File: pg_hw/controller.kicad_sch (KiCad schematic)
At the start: 33 parts, among them J1 USB_C_Receptacle_USB2.0_14P, Q1 SS8050, Q2 SS8050, SW1 SW_MEC_5E, SW2 SW_MEC_5E, U1 BW16, U2 AMS1117-3.3, U3 CH340C, U7 PCF8574A

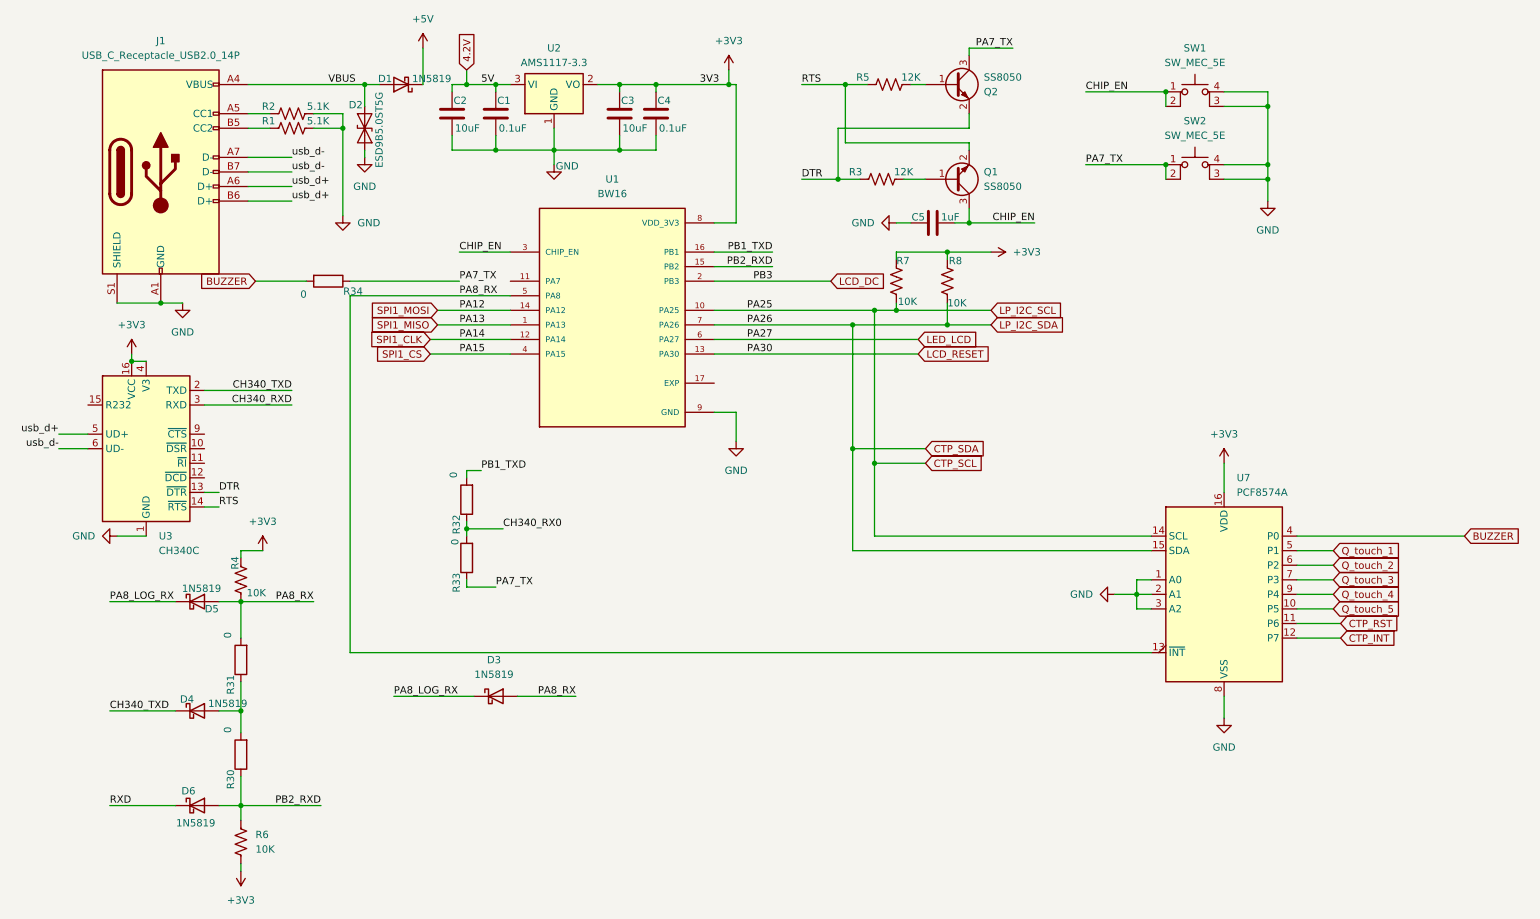
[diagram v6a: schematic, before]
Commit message: charlotte andeh
charlotte andeh
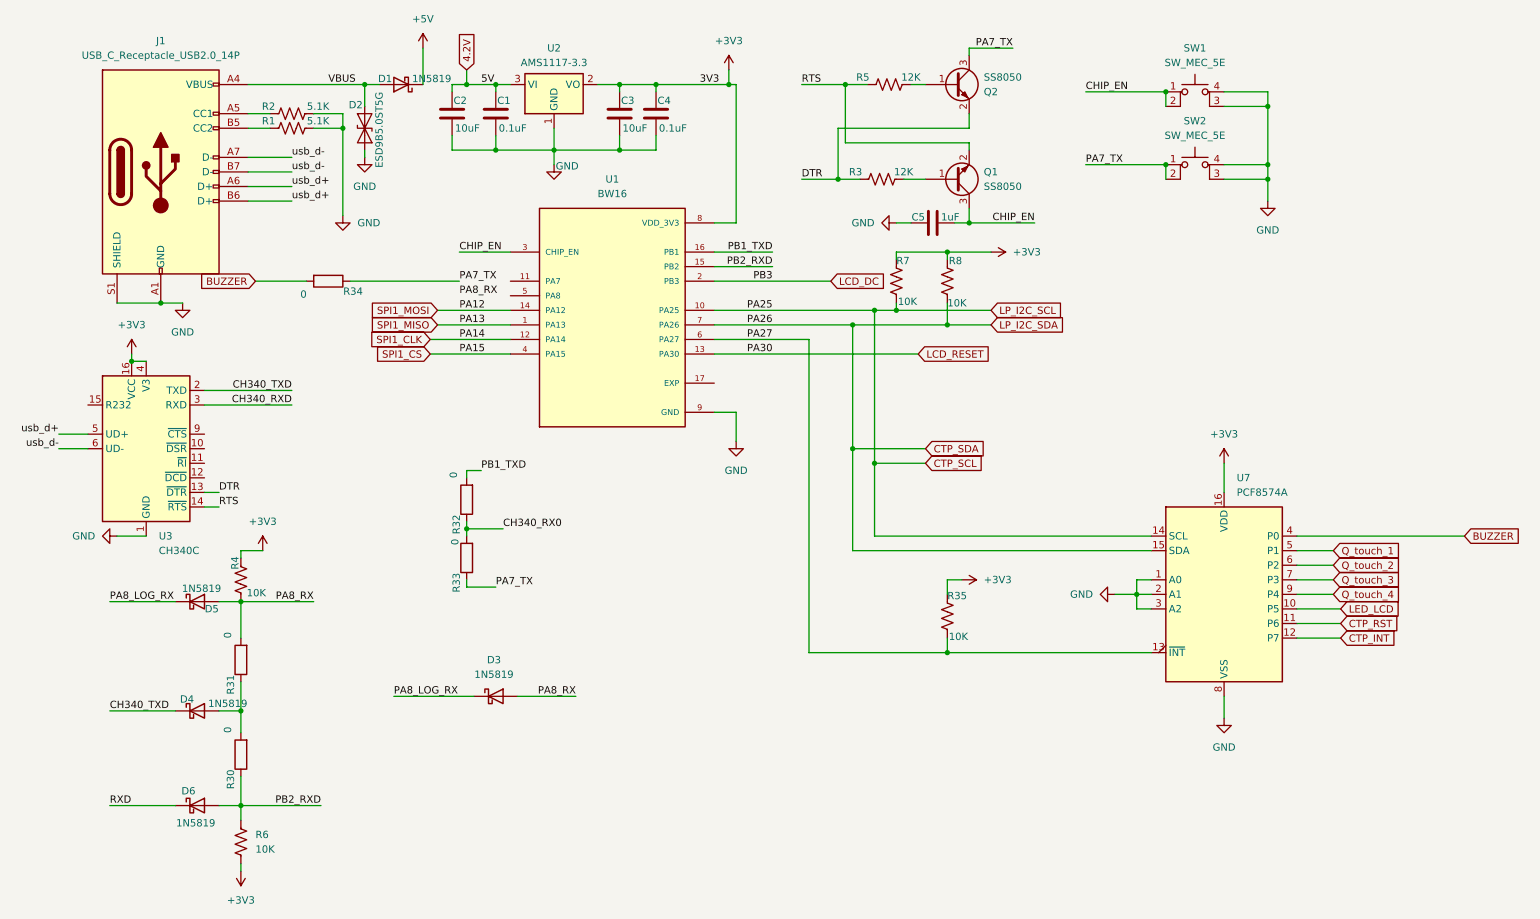
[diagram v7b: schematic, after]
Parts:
- added R35: 10K, Resistor_SMD:R_0402_1005Metric, symbol Device:R_US
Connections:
- net Q_touch_5 is gone; now on net LED_LCD: U7.10 (P5)
- net +3V3: now also R35.1
- net LED_LCD: no longer U1.6 (PA27)
- net PA8_RX: no longer U1.5 (PA8), U7.13 (~{INT})
- new net PA27: R35.2, U1.6 (PA27), U7.13 (~{INT})
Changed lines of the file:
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@@
 	)
 	(junction
+		(at 177.8 130.81)
+		(diameter 0)
+		(color 0 0 0 0)
+	)
+	(junction
 		(at 177.8 60.96)
 		(diameter 0)
@@
 	(wire
 		(pts
-			(xy 137.16 76.2) (xy 172.72 76.2)
+			(xy 137.16 76.2) (xy 153.67 76.2)
 		)
 		(stroke
@@
 	(wire
 		(pts
-			(xy 213.36 130.81) (xy 73.66 130.81)
-		)
-		(stroke
-			(width 0)
-			(type default)
-		)
-	)
-	(wire
-		(pts
 			(xy 201.93 45.72) (xy 215.9 45.72)
 		)
@@
 	(wire
 		(pts
-			(xy 73.66 130.81) (xy 73.66 68.58)
-		)
-		(stroke
-			(width 0)
-			(type default)
-		)
-	)
-	(wire
-		(pts
 			(xy 210.82 118.11) (xy 213.36 118.11)
 		)
@@
 	(wire
 		(pts
+			(xy 180.34 118.11) (xy 177.8 118.11)
+		)
+		(stroke
+			(width 0)
+			(type default)
+		)
+	)
+	(wire
+		(pts
 			(xy 93.98 109.22) (xy 100.33 109.22)
 		)
@@
 	(wire
 		(pts
-			(xy 238.76 123.19) (xy 245.11 123.19)
+			(xy 238.76 123.19) (xy 246.38 123.19)
 		)
 		(stroke
@@
 	(wire
 		(pts
+			(xy 177.8 128.27) (xy 177.8 130.81)
+		)
+		(stroke
+			(width 0)
+			(type default)
+		)
+	)
+	(wire
+		(pts
 			(xy 54.61 152.4) (xy 54.61 157.48)
 		)
@@
 	(wire
 		(pts
-			(xy 96.52 99.06) (xy 93.98 99.06)
+			(xy 153.67 130.81) (xy 153.67 76.2)
 		)
 		(stroke
@@
 	(wire
 		(pts
-			(xy 54.61 140.97) (xy 54.61 144.78)
+			(xy 96.52 99.06) (xy 93.98 99.06)
 		)
 		(stroke
@@
 	(wire
 		(pts
-			(xy 73.66 68.58) (xy 101.6 68.58)
+			(xy 54.61 140.97) (xy 54.61 144.78)
 		)
 		(stroke
@@
 	(wire
 		(pts
+			(xy 177.8 118.11) (xy 177.8 120.65)
+		)
+		(stroke
+			(width 0)
+			(type default)
+		)
+	)
+	(wire
+		(pts
 			(xy 109.22 43.18) (xy 120.65 43.18)
 		)
@@
 	(wire
 		(pts
+			(xy 177.8 130.81) (xy 153.67 130.81)
+		)
+		(stroke
+			(width 0)
+			(type default)
+		)
+	)
+	(wire
+		(pts
 			(xy 181.61 25.4) (xy 181.61 26.67)
 		)
@@
 	(wire
 		(pts
+			(xy 213.36 130.81) (xy 177.8 130.81)
+		)
+		(stroke
+			(width 0)
+			(type default)
+		)
+	)
+	(wire
+		(pts
 			(xy 171.45 31.75) (xy 173.99 31.75)
 		)
@@
 		)
 	)
-	(global_label "Q_touch_5"
-		(shape input)
-		(at 245.11 123.19 0)
-		(fields_autoplaced yes)
-		(effects
-			(font
-				(size 1.27 1.27)
-			)
-			(justify left)
-		)
-		(property "Intersheetrefs" "${INTERSHEET_REFS}"
-			(at 257.8317 123.19 0)
-			(effects
-				(font
-					(size 1.27 1.27)
-				)
-				(justify left)
-				(hide yes)
-			)
-		)
-	)
 	(global_label "CTP_INT"
 		(shape input)
@@
 	(global_label "LED_LCD"
 		(shape input)
-		(at 172.72 76.2 0)
+		(at 246.38 123.19 0)
 		(fields_autoplaced yes)
 		(effects
@@
 		)
 		(property "Intersheetrefs" "${INTERSHEET_REFS}"
-			(at 183.688 76.2 0)
+			(at 257.348 123.19 0)
 			(effects
 				(font
@@
 	)
 	(symbol
+		(lib_id "Device:R_US")
+		(at 177.8 124.46 0)
+		(unit 1)
+		(exclude_from_sim no)
+		(in_bom yes)
+		(on_board yes)
+		(dnp no)
+		(property "Reference" "R35"
+			(at 177.8 120.904 0)
+			(effects
+				(font
+					(size 1.27 1.27)
+				)
+				(justify left)
+			)
+		)
+		(property "Value" "10K"
+			(at 178.054 128.016 0)
+			(effects
+				(font
+					(size 1.27 1.27)
+				)
+				(justify left)
+			)
+		)
+		(property "Footprint" "Resistor_SMD:R_0402_1005Metric"
+			(at 178.816 124.714 90)
+			(effects
+				(font
+					(size 1.27 1.27)
+				)
+				(hide yes)
+			)
+		)
+		(property "Datasheet" "~"
+			(at 177.8 124.46 0)
+			(effects
+				(font
+					(size 1.27 1.27)
+				)
+				(hide yes)
+			)
+		)
+		(property "Description" "Resistor, US symbol"
+			(at 177.8 124.46 0)
+			(effects
+				(font
+					(size 1.27 1.27)
+				)
+				(hide yes)
+			)
+		)
+		(pin "1"
+		)
+		(pin "2"
+		)
+		(instances
+			(project "pg_hw"
+				(path "/98c2be80-c7ca-4fe5-b302-238a0f594199/8ba1f843-15ae-42f6-a267-5fa0b50da669"
+					(reference "R35")
+					(unit 1)
+				)
+			)
+		)
+	)
+	(symbol
 		(lib_id "Device:C")
 		(at 91.44 36.83 0)
@@
 					(unit 1)
 				)
+			)
+		)
+	)
+	(symbol
+		(lib_id "power:+3V3")
+		(at 180.34 118.11 270)
+		(unit 1)
+		(exclude_from_sim no)
+		(in_bom yes)
+		(on_board yes)
+		(dnp no)
+		(fields_autoplaced yes)
+		(property "Reference" "#PWR050"
+			(at 176.53 118.11 0)
+			(effects
+				(font
+					(size 1.27 1.27)
+				)
+				(hide yes)
+			)
+		)
+		(property "Value" "+3V3"
+			(at 184.15 118.1099 90)
+			(effects
+				(font
+					(size 1.27 1.27)
+				)
+				(justify left)
+			)
+		)
+		(property "Footprint" ""
+			(at 180.34 118.11 0)
+			(effects
+				(font
+					(size 1.27 1.27)
+				)
+				(hide yes)
+			)
+		)
+		(property "Datasheet" ""
+			(at 180.34 118.11 0)
+			(effects
+				(font
+					(size 1.27 1.27)
+				)
+				(hide yes)
+			)
+		)
+		(property "Description" "Power symbol creates a global label with name \"+3V3\""
+			(at 180.34 118.11 0)
+			(effects
+				(font
+					(size 1.27 1.27)
+				)
+				(hide yes)
+			)
+		)
+		(pin "1"
+		)
+		(instances
+			(project "pg_hw"
+				(path "/98c2be80-c7ca-4fe5-b302-238a0f594199/8ba1f843-15ae-42f6-a267-5fa0b50da669"
+					(reference "#PWR050")
+					(unit 1)
+				)

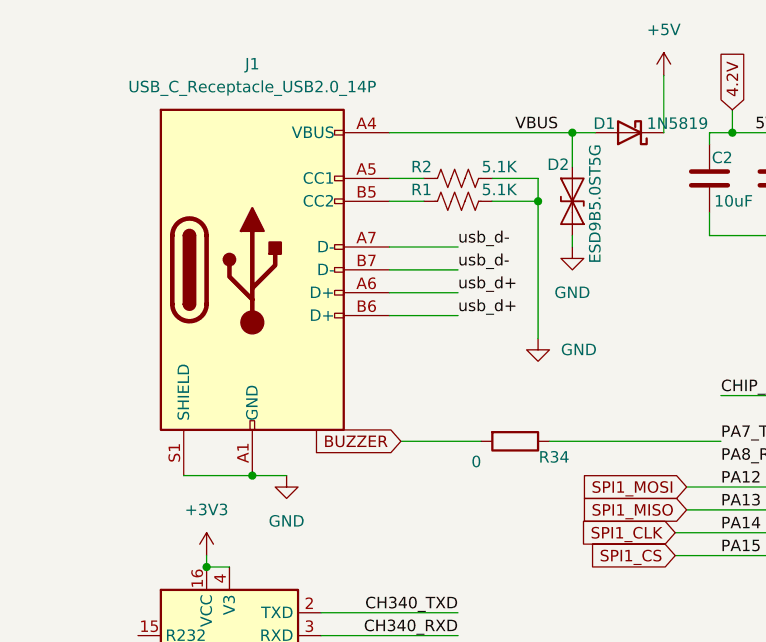
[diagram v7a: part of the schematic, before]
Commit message: usb revision
add some revision
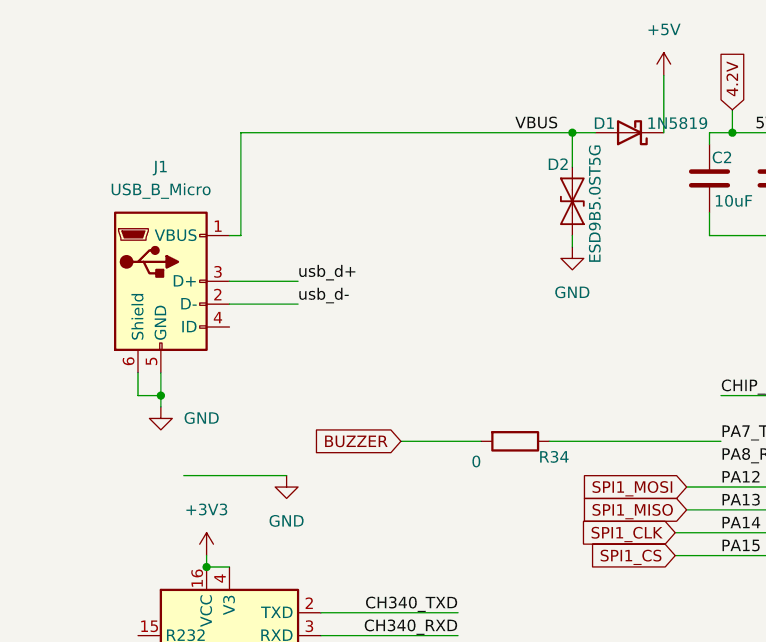
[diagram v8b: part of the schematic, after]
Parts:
- removed J1: USB_C_Receptacle_USB2.0_14P, symbol Connector:USB_C_Receptacle_USB2.0_14P
- removed R1, R2: 5.1K, Resistor_SMD:R_0603_1608Metric, symbol Device:R_US
- added J1: USB_B_Micro, symbol Connector:USB_B_Micro
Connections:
- net GND: now also J1.5 (GND), J1.6 (Shield)
- net VBUS: now also J1.1 (VBUS)
- net usb_d+: now also J1.3 (D+)
- net usb_d-: now also J1.2 (D-)
